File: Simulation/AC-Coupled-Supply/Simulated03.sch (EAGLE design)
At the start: 10 parts, among them X1 TRANSFORMER

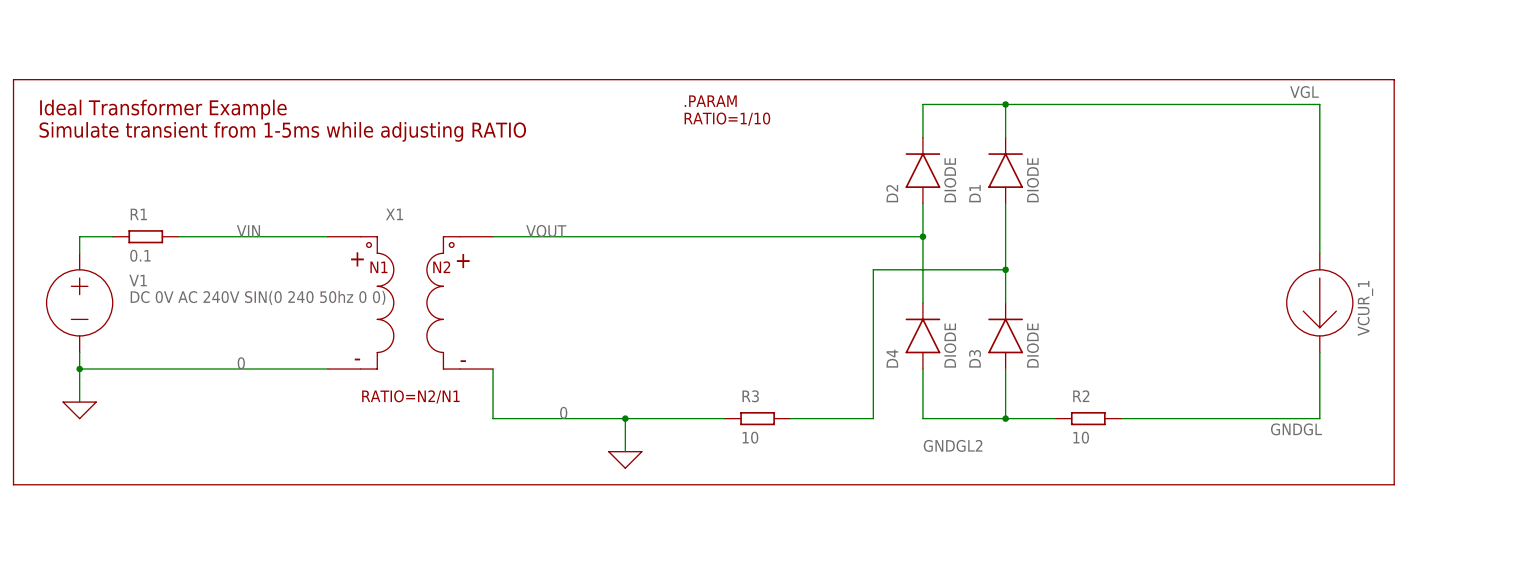
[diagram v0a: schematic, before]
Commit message: zener simulation
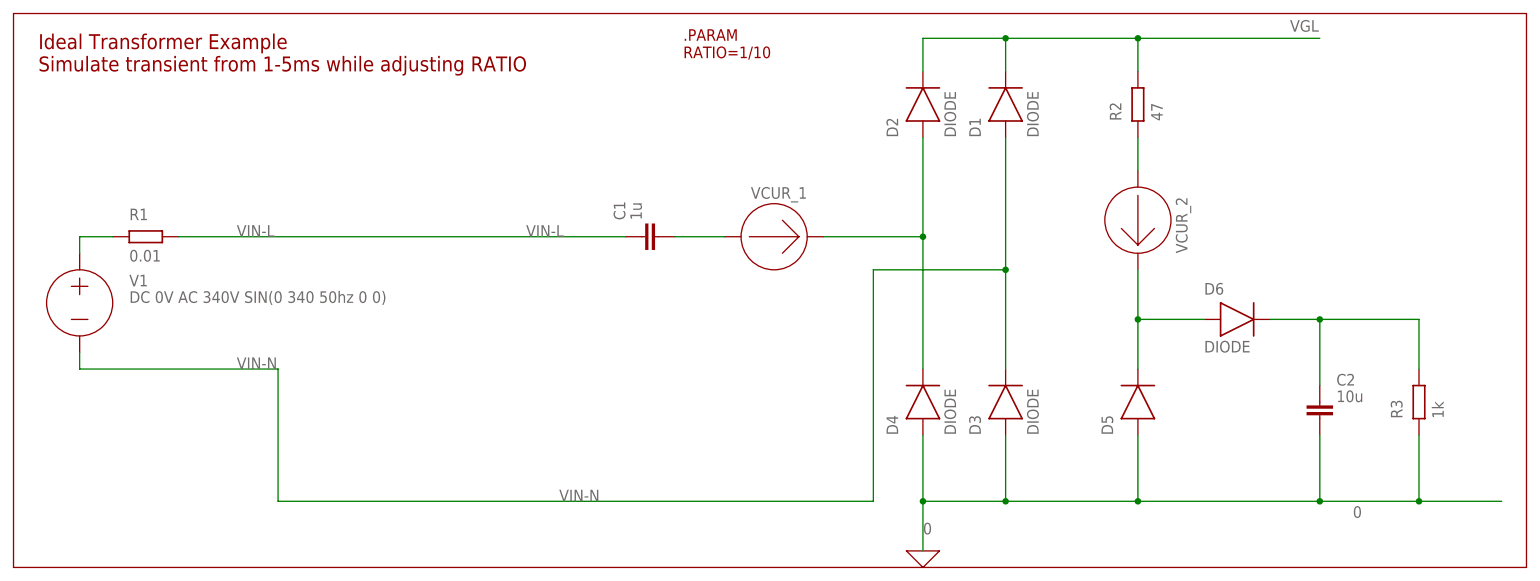
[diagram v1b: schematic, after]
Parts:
- removed X1: TRANSFORMER, ngspice-simulation:TRANSFORMER
- added C1: 1u, ngspice-simulation:C
- added C2: 10u, ngspice-simulation:C
- added D5, D6: DIODE, ngspice-simulation:DIODE
- added VCUR_2: (no value), ngspice-simulation:AMMETER
- R1: value 0.1 -> 0.01
- R2: value 10 -> 47
- R3: value 10 -> 1k
- V1: value DC 0V AC 240V SIN(0 240 50hz 0 0) -> DC 0V AC 340V SIN(0 340 50hz 0 0)
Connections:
- removed net GNDGL: R2.2, VCUR_1.-
- removed net GNDGL2: D3.A, D4.A, R2.1
- removed net VIN: R1.2, X1.P$1
- removed net VOUT: D2.A, D4.C, X1.P$3
- new net N$1: R2.1, VCUR_2.+
- new net N$3: D2.A, D4.C, VCUR_1.-
- new net VIN-L: C1.1, R1.2
- new net VIN-N: D1.A, D3.C, V1.-
- new net VPREREG: D5.C, D6.A, VCUR_2.-
- new net VREG: C2.1, D6.C, R3.2
- net 0: now also C2.2, D3.A, D4.A, D5.A; no longer V1.-, X1.P$2, X1.P$4
- net N$4: now also C1.2, VCUR_1.+; no longer D1.A, D3.C, R3.2
- net VGL: now also R2.2; no longer VCUR_1.+
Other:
- moved on the sheet: D1, D2, D3, D4, R2, R3, VCUR_1
